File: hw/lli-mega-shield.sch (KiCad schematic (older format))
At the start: 28 parts, among them J1 DB25, P1 Enable, Q1 NPN, U1 APC220, U2 LM35, U5 ADIS16405, U6 R-78B5.0-1.5, U7 UP500/UP501

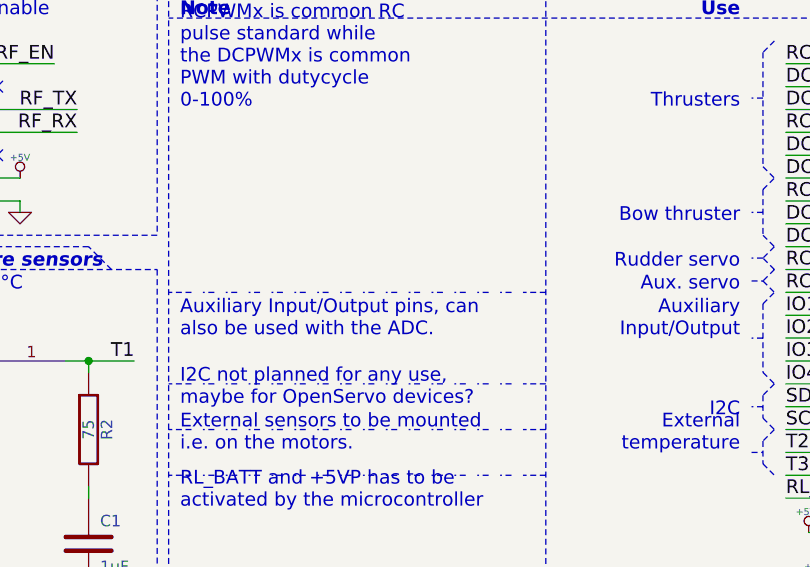
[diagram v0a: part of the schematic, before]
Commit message: Updated a note
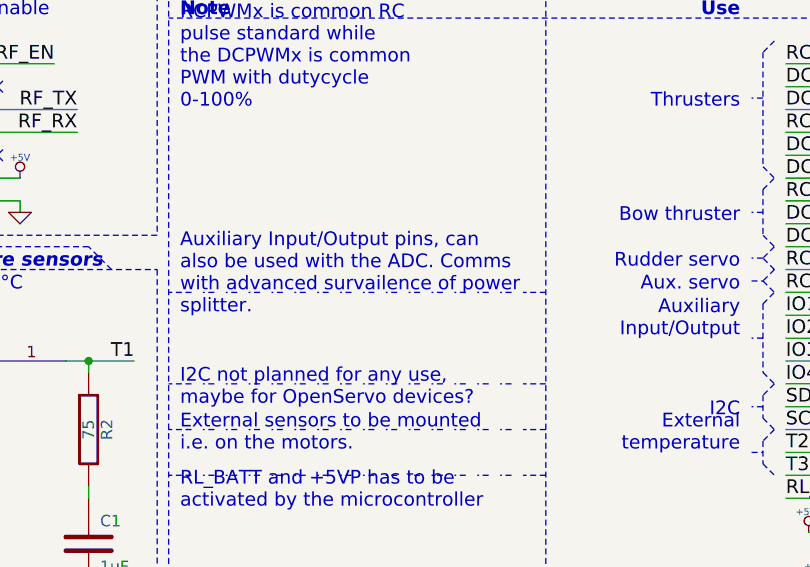
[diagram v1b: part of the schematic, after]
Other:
- note added: "Auxiliary Input/Output pins, can\nalso be used with the ADC. Comms\nwith advanced survailence of power\nsplitter."
- note removed: "Auxiliary Input/Output pins, can\nalso be used with the ADC."
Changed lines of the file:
@@
-EESchema Schematic File Version 2  date søn 30 sep 2012 19:45:06 CEST
+EESchema Schematic File Version 2  date søn 30 sep 2012 20:16:28 CEST
 LIBS:power
 LIBS:device
@@
 Text Notes 8150 6950 0    60   ~ 0
 TODO:\n* Differentiate between arduino 5V and DC-DC 5V\n* Differentiate between Battery direct and relayed battery supply
-Text Notes 2300 2200 0    60   ~ 0
-Auxiliary Input/Output pins, can\nalso be used with the ADC.
+Text Notes 2300 2100 0    60   ~ 0
+Auxiliary Input/Output pins, can\nalso be used with the ADC. Comms\nwith advanced survailence of power\nsplitter.
 Text Label 4950 2100 0    60   ~ 0
 IO1
